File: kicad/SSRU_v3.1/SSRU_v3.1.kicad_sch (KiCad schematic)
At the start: 83 parts, among them J1 AVR-ISP-6, J2 Conn_01x24, J3 Conn_02x03_Odd_Even, J31 Conn_01x04, J6 Conn_02x03_Odd_Even, SW1 SW_Push, U1 MCP2515-xSO, U10 TJA1051T, U11 TCA9517D, U12 TJA1051T, U13 CH340N, U2 ATmega328P-A, U4 LM2576S-5, U5 AMS1117-3.3, U7 MCP2515-xSO, U8 74LVC1G17, U9 MT3608/SDB628, Y1 16MHz, Y3 16MHz, Y4 16MHz

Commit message: ssru3.1 pcb edgec ut
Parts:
- removed C9: 22uF, RMC_Capacitor:C_0805_2012Metric_Pad1.18x1.45mm_HandSolder_L, symbol Device:C_Polarized
- removed H3, H4: MountingHole, MountingHole:MountingHole_3.2mm_M3, symbol Mechanical:MountingHole
- removed J1: AVR-ISP-6, Connector_PinHeader_2.54mm:PinHeader_2x03_P2.54mm_Vertical, symbol Connector:AVR-ISP-6
- removed J6: Conn_02x03_Odd_Even, symbol Connector_Generic:Conn_02x03_Odd_Even
- added C20: 22uF, RMC_Capacitor:C_0805_2012Metric_Pad1.18x1.45mm_HandSolder_L, symbol Device:C_Polarized
- added J1, J5: Conn_01x03, Connector_PinHeader_2.54mm:PinHeader_1x03_P2.54mm_Vertical, symbol Connector_Generic:Conn_01x03
- added J4: AVR-ISP-6, Connector_PinHeader_2.54mm:PinHeader_2x03_P2.54mm_Vertical, symbol Connector:AVR-ISP-6
- added R1, R2, R3, R6, R7, R8: 1M, RMC_Resistor:R_0805_2012Metric_Pad1.20x1.40mm_HandSolder_L, symbol Device:R
- C32, C33: footprint RMC_Capacitor:CP_EIA-3528-15_AVX-H_Pad1.50x2.35mm_HandSolder_RMC -> RMC_Capacitor:C_0805_2012Metric_Pad1.18x1.45mm_HandSolder_L
- J2: footprint (none) -> RMC_Connnector:HD241_24pin
- J3: footprint (none) -> Connector_PinHeader_2.54mm:PinHeader_2x03_P2.54mm_Vertical
- L2: footprint Inductor_SMD:L_Wuerth_HCI-5040 -> RMC_Inductor:L_10.4x10.4_H4.8_handsolder
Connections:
- net +12V: no longer J2.2 (Pin_2)
- net +24V: now also J2.14 (Pin_14)
- net +5V: now also J2.9 (Pin_9), J4.2 (VCC); no longer J2.10 (Pin_10), J2.14 (Pin_14)
- net CAN1+: now also J2.4 (Pin_4), J2.6 (Pin_6); no longer J2.5 (Pin_5), J2.7 (Pin_7)
- net CAN1-: now also J2.3 (Pin_3), J2.5 (Pin_5); no longer J2.4 (Pin_4), J2.6 (Pin_6)
- net CAN2+: now also J2.8 (Pin_8); no longer J2.9 (Pin_9)
- net CAN2-: now also J2.7 (Pin_7); no longer J2.8 (Pin_8)
- net DS18B20: now also J2.13 (Pin_13); no longer J2.16 (Pin_16)
- net ENCODER_A: now also J3.5 (Pin_5), R8.2
- net ENCODER_B: now also J3.6 (Pin_6), R7.2
- net FLOW_IN: now also J3.2 (Pin_2), J5.2 (Pin_2), R3.2; no longer J3.3 (Pin_3), U8.2
- net FLOW_OUT: now also J5.1 (Pin_1)
- net GND: now also J2.2 (Pin_2), C20.2, J1.3 (Pin_3), J4.6 (GND), R1.1, R2.1, R3.1, R6.1, R7.1, R8.1; no longer J2.15 (Pin_15), J2.3 (Pin_3)
- net MISO: now also J4.1 (MISO)
- net MOSI: now also J4.4 (MOSI)
- net POT1_IN: now also J2.10 (Pin_10), R1.2; no longer J2.11 (Pin_11)
- net POT2_IN: now also J2.11 (Pin_11), R2.2; no longer J2.13 (Pin_13)
- net PUMP_NTC_50k: now also R6.2
- net PUMP_PWM: now also J1.1 (Pin_1); no longer J3.5 (Pin_5)
- net RST: now also J4.5 (~{RST})
- net SCK: now also J4.3 (SCK)
- net j1: now also J3.3 (Pin_3); no longer J3.2 (Pin_2)
- net j3: now also J1.2 (Pin_2); no longer J3.6 (Pin_6)
- net at C10.2, F1.2, U5.2 (VO): now also C20.1
- new net: J5.3 (Pin_3), U8.2
- new net BRAKE_TEMP1: J2.15 (Pin_15)
- new net BRAKE_TEMP2: J2.16 (Pin_16)
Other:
- sheet current to voltage ports: added BRAKE_TEMP_IN1, BRAKE_TEMP_IN2; removed none
- moved on the sheet: C19, C30, J3, U8

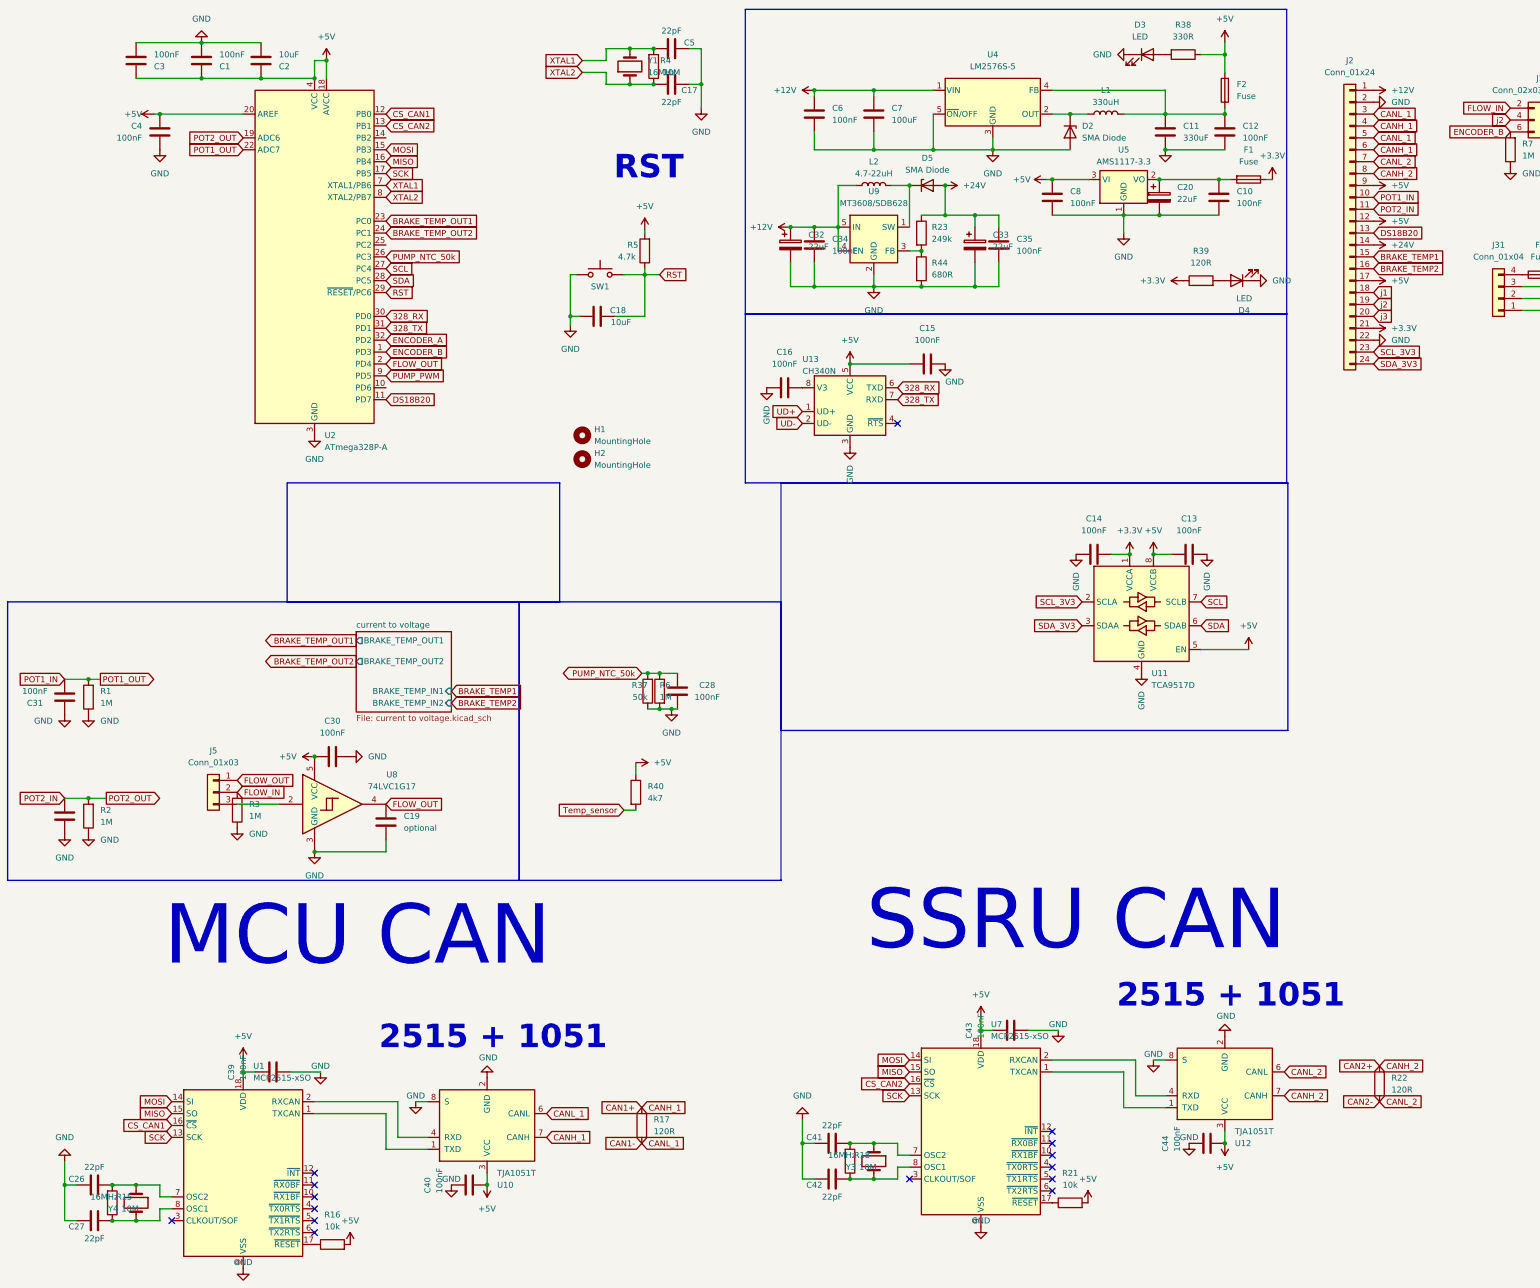
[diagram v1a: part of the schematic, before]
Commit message: SSRU v3.1 updates
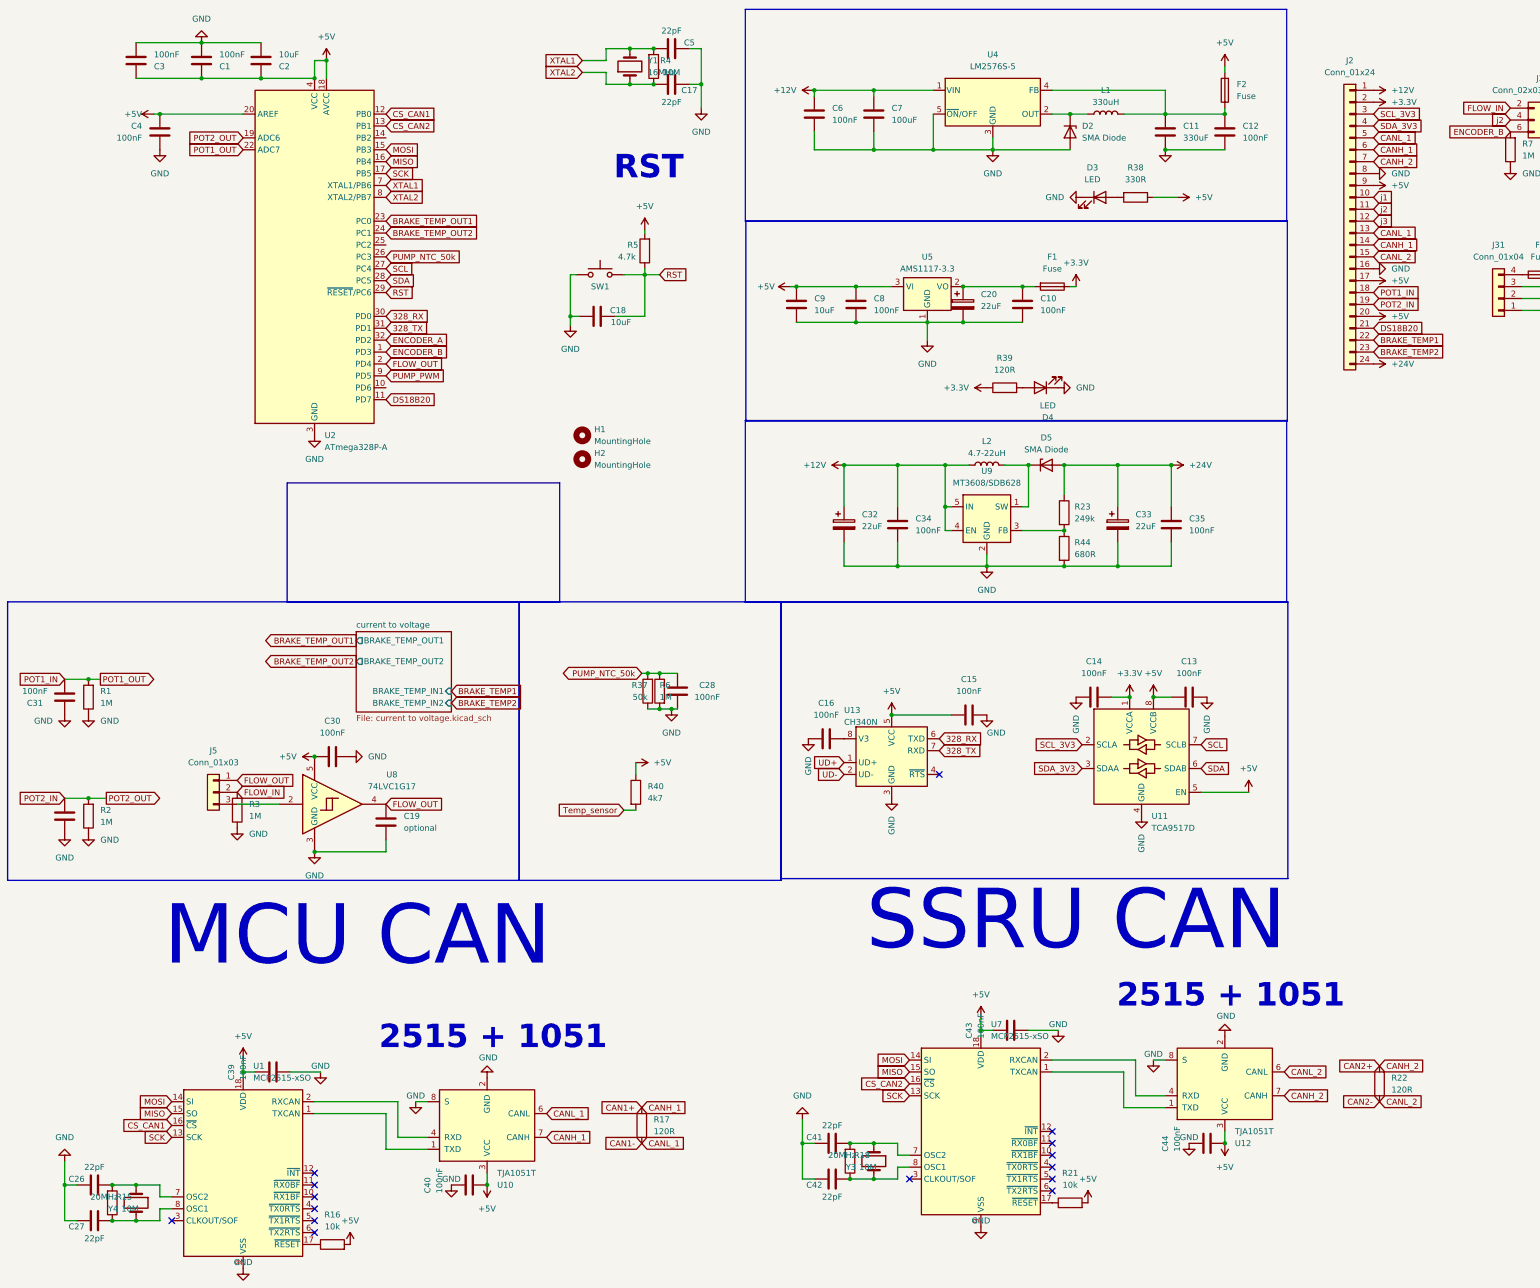
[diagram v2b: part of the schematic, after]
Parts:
- added C9: 10uF, RMC_Capacitor:C_0805_2012Metric_Pad1.18x1.45mm_HandSolder_L, symbol Device:C
- J5: footprint Connector_PinHeader_2.54mm:PinHeader_1x03_P2.54mm_Vertical -> Jumper:SolderJumper-3_P1.3mm_Open_Pad1.0x1.5mm
- L2: footprint RMC_Inductor:L_10.4x10.4_H4.8_handsolder -> Inductor_SMD:L_Sunlord_SWPA5040S
- U11: footprint Package_SO:SOIC-8_3.9x4.9mm_P1.27mm -> RMC_SO:SOIC-8_3.9x4.9mm_P1.27mm_RMC_Handsolder
- U13: footprint Package_SO:SOP-8_3.9x4.9mm_P1.27mm -> RMC_SO:SOIC-8_3.9x4.9mm_P1.27mm_RMC_Handsolder
- Y3, Y4: value 16MHz -> 20MHz
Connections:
- net +24V: now also J2.24 (Pin_24); no longer J2.14 (Pin_14)
- net +3.3V: now also J2.2 (Pin_2); no longer J2.21 (Pin_21)
- net +5V: now also J2.20 (Pin_20), C9.2; no longer J2.12 (Pin_12)
- net BRAKE_TEMP1: now also J2.22 (Pin_22); no longer J2.15 (Pin_15)
- net BRAKE_TEMP2: now also J2.23 (Pin_23); no longer J2.16 (Pin_16)
- net CAN1+: now also J2.14 (Pin_14); no longer J2.4 (Pin_4)
- net CAN1-: now also J2.13 (Pin_13); no longer J2.3 (Pin_3)
- net CAN2+: now also J2.7 (Pin_7); no longer J2.8 (Pin_8)
- net CAN2-: now also J2.15 (Pin_15); no longer J2.7 (Pin_7)
- net DS18B20: now also J2.21 (Pin_21); no longer J2.13 (Pin_13)
- net GND: now also J2.16 (Pin_16), J2.8 (Pin_8), C9.1; no longer J2.2 (Pin_2), J2.22 (Pin_22)
- net POT1_IN: now also J2.18 (Pin_18); no longer J2.10 (Pin_10)
- net POT2_IN: now also J2.19 (Pin_19); no longer J2.11 (Pin_11)
- net SCL_3V3: now also J2.3 (Pin_3); no longer J2.23 (Pin_23)
- net SDA_3V3: now also J2.4 (Pin_4); no longer J2.24 (Pin_24)
- net j1: now also J2.10 (Pin_10); no longer J2.18 (Pin_18)
- net j2: now also J2.11 (Pin_11); no longer J2.19 (Pin_19)
- net j3: now also J2.12 (Pin_12); no longer J2.20 (Pin_20)
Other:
- moved on the sheet: C10, C13, C14, C15, C16, C20, C32, C33, C34, C35, C8, D3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
